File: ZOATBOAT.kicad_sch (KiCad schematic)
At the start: 131 parts, among them SW1 SW_Push_45deg, SW10 SW_Push_45deg, SW11 SW_Push_45deg, SW12 SW_Push_45deg, SW13 SW_Push_45deg, SW14 SW_Push_45deg, SW15 SW_Push_45deg, SW16 SW_Push_45deg, SW17 SW_Push_45deg, SW18 SW_Push_45deg, SW19 SW_Push_45deg, SW2 SW_Push_45deg, SW20 SW_Push_45deg, SW21 SW_Push_45deg, SW22 SW_Push_45deg, SW23 SW_Push_45deg, SW24 SW_Push_45deg, SW25 SW_Push_45deg, SW26 SW_Push_45deg, SW27 SW_Push_45deg, SW28 SW_Push_45deg, SW29 SW_Push_45deg, SW3 SW_Push_45deg, SW30 SW_Push_45deg, SW31 SW_Push_45deg, SW32 SW_Push_45deg, SW33 SW_Push_45deg, SW34 SW_Push_45deg, SW35 SW_Push_45deg, SW36 SW_Push_45deg, SW37 SW_Push_45deg, SW38 SW_Push_45deg, SW39 SW_Push_45deg, SW4 SW_Push_45deg, SW40 SW_Push_45deg, SW41 SW_Push_45deg, SW42 SW_Push_45deg, SW43 SW_Push_45deg, SW44 SW_Push_45deg, SW45 SW_Push_45deg, SW46 SW_Push_45deg, SW47 SW_Push_45deg, SW48 SW_Push_45deg, SW49 SW_Push_45deg, SW5 SW_Push_45deg, SW50 SW_Push_45deg, SW51 SW_Push_45deg, SW52 SW_Push_45deg, SW53 SW_Push_45deg, SW54 SW_Push_45deg, SW55 SW_Push_45deg, SW56 SW_Push_45deg, SW57 SW_Push_45deg, SW58 SW_Push_45deg, SW59 SW_Push_45deg, SW6 SW_Push_45deg, SW60 SW_Push_45deg, SW61 SW_Push_45deg, SW62 SW_Push_45deg, SW63 SW_Push_45deg, SW64 SW_Push_45deg, SW65 RotaryEncoder_Switch, SW66 RotaryEncoder_Switch, SW7 SW_Push_45deg, SW8 SW_Push_45deg, SW9 SW_Push_45deg

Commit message: added footprints to schematics
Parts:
- SW1, SW11, SW13, SW15, SW17, SW19, SW2, SW21, SW23, SW25, SW27, SW29, SW3, SW31, SW33, SW35, SW37, SW39, SW4, SW41, SW43, SW45, SW47, SW49, SW51, SW53, SW55, SW57, SW59, SW61, SW63, SW9: footprint Button_Switch_THT:SW_NKK_GW12LJP -> ScottoKeebs_Hotswap:Hotswap_MX_1.00u
- SW10, SW12, SW14, SW16, SW18, SW20, SW22, SW24, SW26, SW28, SW30, SW32, SW34, SW36, SW38, SW40, SW42, SW44, SW46, SW48, SW5, SW50, SW52, SW54, SW56, SW58, SW6, SW60, SW62, SW64, SW7, SW8: footprint (none) -> ScottoKeebs_Hotswap:Hotswap_MX_1.00u
- SW65, SW66: footprint Button_Switch_SMD:Nidec_Copal_CAS-120A -> Rotary_Encoder:RotaryEncoder_Alps_EC11E-Switch_Vertical_H20mm

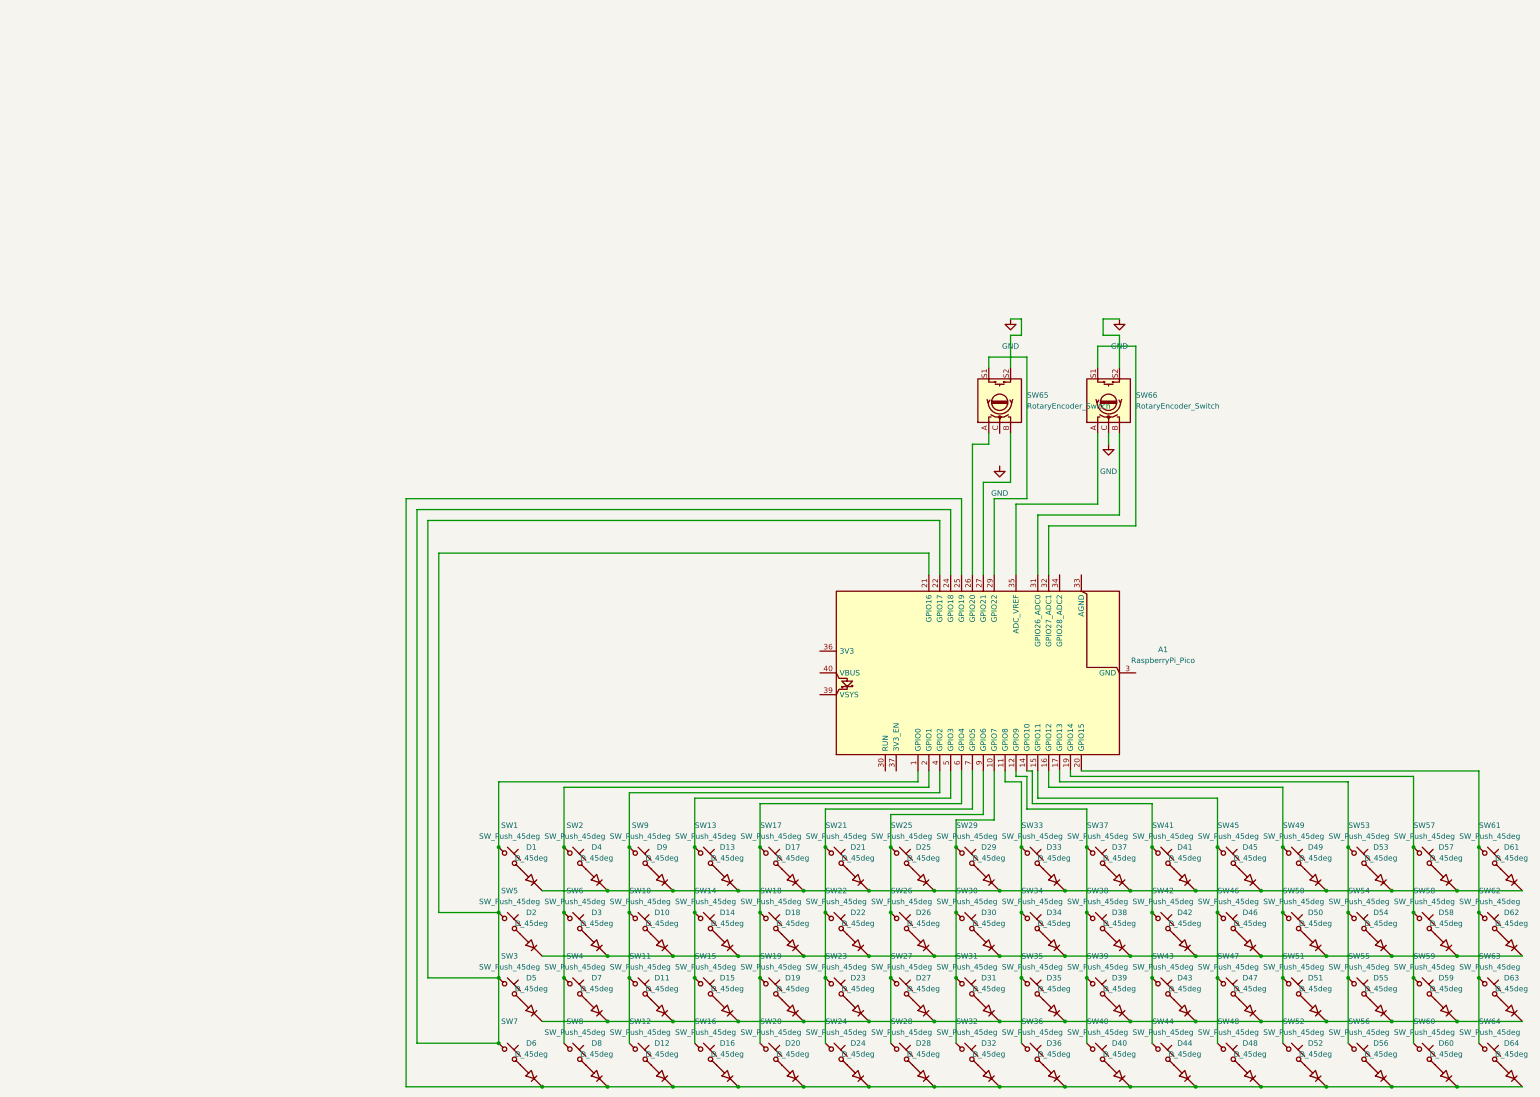
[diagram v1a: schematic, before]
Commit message: redid the entire schematic because i did it wrong
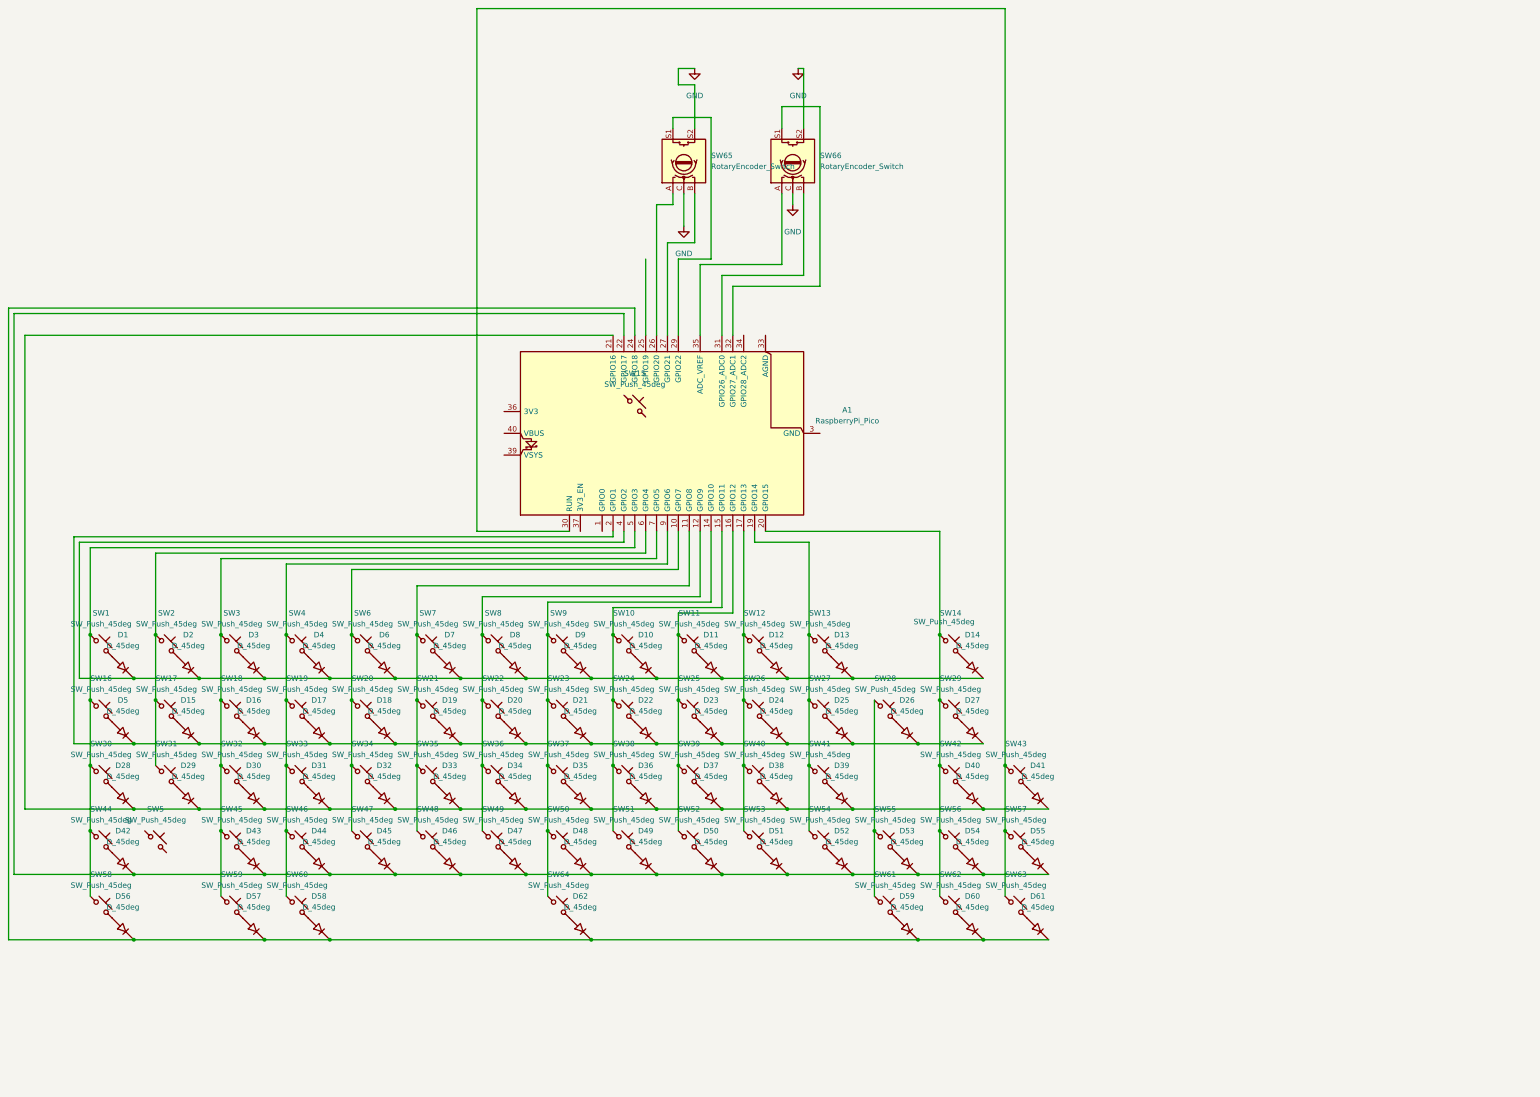
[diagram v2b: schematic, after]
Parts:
- removed D63, D64: D_45deg, Diode_THT:D_DO-35_SOD27_P7.62mm_Horizontal, symbol Device:D_45deg
- D1, D10, D11, D12, D13, D14, D15, D16, D17, D18, D19, D2, D20, D21, D22, D23, D24, D25, D26, D27, D28, D29, D3, D30, D31, D32, D33, D34, D35, D36, D37, D38, D39, D4, D40, D41, D42, D43, D44, D45, D46, D47, D48, D49, D5, D50, D51, D52, D53, D54, D55, D56, D57, D58, D59, D6, D60, D61, D62, D7, D8, D9: footprint Diode_THT:D_DO-35_SOD27_P7.62mm_Horizontal -> Diode_THT:D_A-405_P7.62mm_Horizontal
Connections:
- net GND: now also SW65.C
- net at D48.2 (A): now also SW50.2; no longer SW48.2
- net at SW42.2: now also D40.2 (A); no longer D42.2 (A)
- net at D36.2 (A): now also SW38.2; no longer SW36.2
- net at SW7.2: now also D7.2 (A); no longer D6.2 (A)
- net at D33.2 (A): now also SW35.2; no longer SW33.2
- net at D19.2 (A): now also SW21.2; no longer SW19.2
- net at SW49.2: now also D47.2 (A); no longer D49.2 (A)
- net at D2.2 (A): now also SW2.2; no longer SW5.2
- net at D53.2 (A): now also SW55.2; no longer SW53.2
- net at D57.2 (A): now also SW59.2; no longer SW57.2
- net at D50.2 (A): now also SW52.2; no longer SW50.2
- net at D17.2 (A): now also SW19.2; no longer SW17.2
- net at D51.2 (A): now also SW53.2; no longer SW51.2
- net at SW43.2: now also D41.2 (A); no longer D43.2 (A)
- net at SW27.2: now also D25.2 (A); no longer D27.2 (A)
- net at D18.2 (A): now also SW20.2; no longer SW18.2
- net at SW46.2: now also D44.2 (A); no longer D46.2 (A)
- net at D61.2 (A): now also SW63.2; no longer SW61.2
- net at SW28.2: now also D26.2 (A); no longer D28.2 (A)
- net at D24.2 (A): now also SW26.2; no longer SW24.2
- net at SW47.2: now also D45.2 (A); no longer D47.2 (A)
- net at SW44.2: now also D42.2 (A); no longer D44.2 (A)
- net at SW62.2: now also D60.2 (A); no longer D62.2 (A)
- net at D20.2 (A): now also SW22.2; no longer SW20.2
- net at D35.2 (A): now also SW37.2; no longer SW35.2
- net at D55.2 (A): now also SW57.2; no longer SW55.2
- net at D38.2 (A): now also SW40.2; no longer SW38.2
- net at SW25.2: now also D23.2 (A); no longer D25.2 (A)
- net at D58.2 (A): now also SW60.2; no longer SW58.2
- net at D4.2 (A): now also SW4.2; no longer SW2.2
- net at D32.2 (A): now also SW34.2; no longer SW32.2
- net at SW56.2: now also D54.2 (A); no longer D56.2 (A)
- net at D37.2 (A): now also SW39.2; no longer SW37.2
- net at D3.2 (A): now also SW3.2; no longer SW6.2
- net at SW23.2: now also D21.2 (A); no longer D23.2 (A)
- net at SW15.2: no longer D15.2 (A)
- net at D5.2 (A): now also SW16.2; no longer SW3.2
- net at SW45.2: now also D43.2 (A); no longer D45.2 (A)
- net at SW54.2: now also D52.2 (A); no longer D54.2 (A)
- net at D22.2 (A): now also SW24.2; no longer SW22.2
- net at SW41.2: now also D39.2 (A); no longer D41.2 (A)
- net at D16.2 (A): now also SW18.2; no longer SW16.2
- net at SW64.2: now also D62.2 (A)
- net at D31.2 (A): now also SW33.2; no longer SW31.2
- net at SW30.2: now also D28.2 (A); no longer D30.2 (A)
- net at A1.30 (RUN): now also SW43.1, SW57.1, SW63.1
- net at D34.2 (A): now also SW36.2; no longer SW34.2
- net at D59.2 (A): now also SW61.2; no longer SW59.2
- net at D29.2 (A): now also SW31.2; no longer SW29.2
- new net: SW28.1, SW55.1, SW61.1
- new net: A1.16 (GPIO12), SW11.1, SW25.1, SW39.1, SW52.1
- new net: A1.20 (GPIO15), SW14.1, SW29.1, SW42.1, SW56.1, SW62.1
- new net: A1.22 (GPIO17), D42.1 (K), D43.1 (K), D44.1 (K), D45.1 (K), D46.1 (K), D47.1 (K), D48.1 (K), D49.1 (K), D50.1 (K), D51.1 (K), D52.1 (K), D53.1 (K), D54.1 (K), D55.1 (K)
- new net: A1.4 (GPIO2), D1.1 (K), D10.1 (K), D11.1 (K), D12.1 (K), D13.1 (K), D14.1 (K), D2.1 (K), D3.1 (K), D4.1 (K), D6.1 (K), D7.1 (K), D8.1 (K), D9.1 (K)
- new net: A1.10 (GPIO7), SW20.1, SW34.1, SW47.1, SW6.1
- new net: A1.17 (GPIO13), SW12.1, SW26.1, SW40.1, SW53.1
- new net: A1.24 (GPIO18), D56.1 (K), D57.1 (K), D58.1 (K), D59.1 (K), D60.1 (K), D61.1 (K), D62.1 (K)
- new net: A1.15 (GPIO11), SW10.1, SW24.1, SW38.1, SW51.1
- new net: A1.21 (GPIO16), D28.1 (K), D29.1 (K), D30.1 (K), D31.1 (K), D32.1 (K), D33.1 (K), D34.1 (K), D35.1 (K), D36.1 (K), D37.1 (K), D38.1 (K), D39.1 (K), D40.1 (K), D41.1 (K)
- new net: A1.19 (GPIO14), SW13.1, SW27.1, SW41.1, SW54.1
- new net: A1.2 (GPIO1), D15.1 (K), D16.1 (K), D17.1 (K), D18.1 (K), D19.1 (K), D20.1 (K), D21.1 (K), D22.1 (K), D23.1 (K), D24.1 (K), D25.1 (K), D26.1 (K), D27.1 (K), D5.1 (K)
- new net: A1.14 (GPIO10), SW23.1, SW37.1, SW50.1, SW64.1, SW9.1
- new net: A1.11 (GPIO8), SW21.1, SW35.1, SW48.1, SW7.1
- new net: A1.12 (GPIO9), SW22.1, SW36.1, SW49.1, SW8.1
- new net: A1.7 (GPIO5), SW18.1, SW3.1, SW32.1, SW45.1, SW59.1
- new net: D30.2 (A), SW32.2
- new net: A1.6 (GPIO4), SW17.1, SW2.1, SW31.1
- new net: A1.9 (GPIO6), SW19.1, SW33.1, SW4.1, SW46.1, SW60.1
- new net: A1.5 (GPIO3), SW1.1, SW16.1, SW30.1, SW44.1, SW58.1
- new net: D56.2 (A), SW58.2
- new net: D46.2 (A), SW48.2
- new net: D15.2 (A), SW17.2
- new net: D49.2 (A), SW51.2
- new net: D27.2 (A), SW29.2
- new net: D6.2 (A), SW6.2
- now unconnected: A1.1 (GPIO0), A1.25 (GPIO19), SW15.1, SW5.1
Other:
- moved on the sheet: A1, SW5, SW65, SW66
